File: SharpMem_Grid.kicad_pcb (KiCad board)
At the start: 2 copper layers, 45 x 36 mm, 33 parts, among them J1 CONN_01X05, J2 CONN_01X01, J3 CONN_01X01, P1 USB_B, P2 CONN_02X04, SW1 PTS810_SJK_250_SMTR_LFS, SW2 PTS810_SJK_250_SMTR_LFS, U1 25LC_EEPROM, U2 Schmitt_Inverter_Single, U3 PIC32MX250F128B-I/SS, Y1 ECS-080-18-23G-JGN-TR

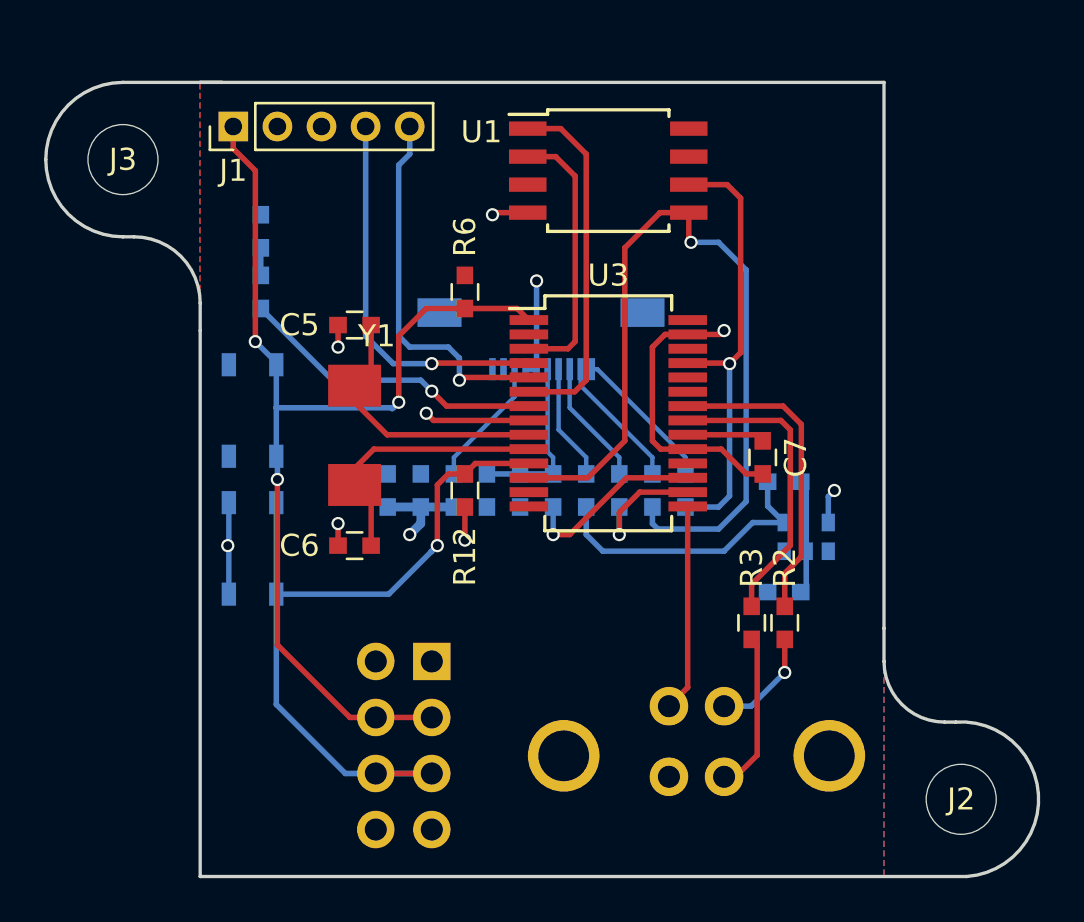
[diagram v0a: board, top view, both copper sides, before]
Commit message: redesighn for itp camp
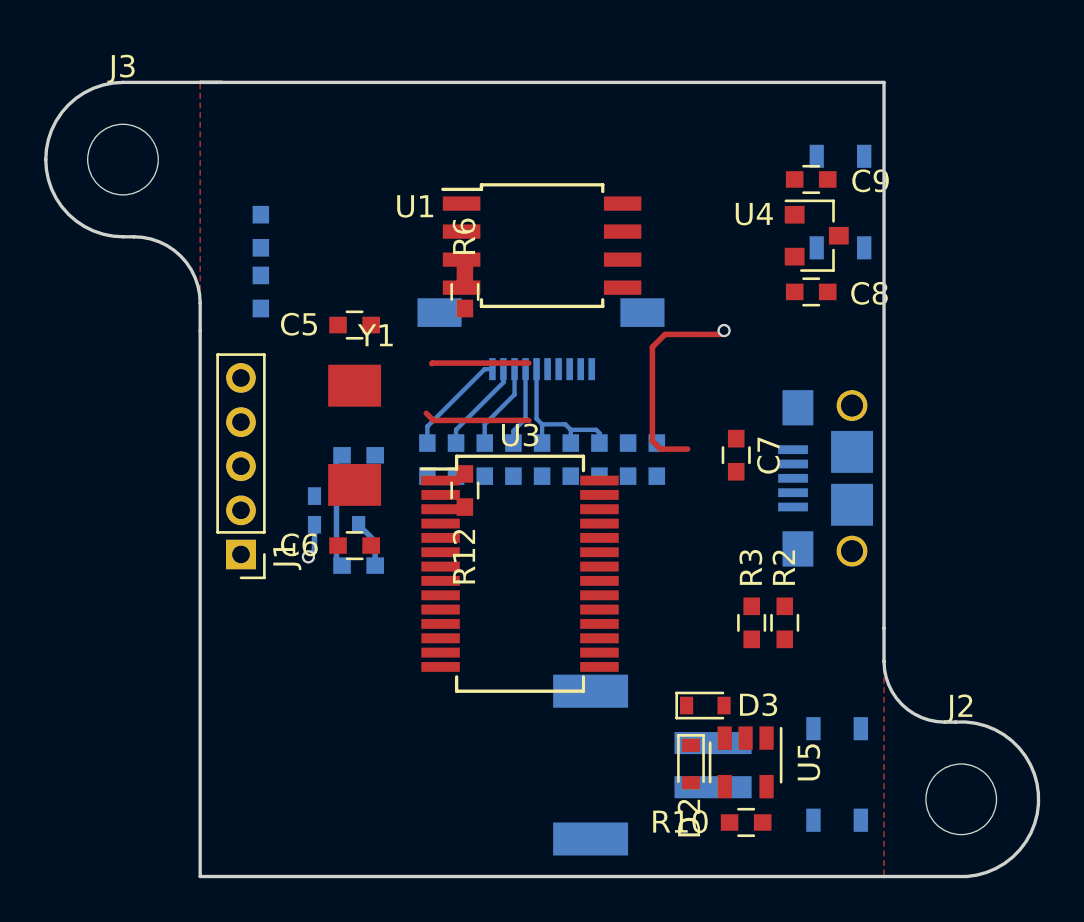
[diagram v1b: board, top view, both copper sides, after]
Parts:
- removed P1: USB_B, Solutions:USB_B_VERTICAL
- removed P2: CONN_02X04, Pin_Headers:Pin_Header_Straight_2x04_Pitch2.54mm
- added BT1: Battery_Cell, Solutions:4UCON-0217-20519, B.Cu at (184.8, 109.7)
- added C8: 1uF, Capacitors_SMD:C_0603, F.Cu at (189.2, 88.2)
- added C9: 1uF, Capacitors_SMD:C_0603, F.Cu at (189.2, 83.2)
- added D2: DIODE, Diodes_SMD:D_0603, F.Cu at (183.8, 109.7)
- added D3: DIODE, Diodes_SMD:D_0603, F.Cu at (184.4, 107.0)
- added J4: USB_B_Micro, Solutions:10118193_microUSB, B.Cu at (191.1, 96.7)
- added U4: TLV76033DBZR, TO_SOT_Packages_SMD:SOT-23, F.Cu at (189.4, 85.7)
- added U5: MCP73831-2-OT, TO_SOT_Packages_SMD:SOT-23-5, F.Cu at (186.2, 109.6)
- J2, J3: footprint Solutions:NPT_125mil -> Mounting_Holes:MountingHole_3.2mm_M3
- R10: moved to F.Cu
- R13: value 10K -> 220R
- R4, R5, R7, R8, R9: value 220 -> 220R
- moved SW2 28.4 mm to (190.0, 109.2)
- moved SW1 28.3 mm to (190.2, 83.3)
- moved U2 21.3 mm to (167.7, 98.2), turned to 270 degrees
- moved C1 20.3 mm to (168.7, 95.7), turned to 180 degrees
- moved R10 20.1 mm to (186.2, 112.3), turned to 180 degrees
- moved R1 19.7 mm to (168.7, 100.7), turned to 0 degrees
- moved J1 19.4 mm to (163.3, 100.2), turned to 180 degrees
- moved C2 12.3 mm to (182.2, 95.8), turned to 270 degrees
- moved R4 11.8 mm to (171.8, 95.8)
- moved C3 9.50 mm to (180.9, 95.8), turned to 270 degrees
- moved R5 9.01 mm to (173.1, 95.8)
- moved U3 8.30 mm to (176.0, 101.0)
- moved R7 6.26 mm to (174.4, 95.8)
- moved C4 5.29 mm to (179.6, 95.8)
- moved U1 4.53 mm to (177.0, 86.2)
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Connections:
- D1 pad 2: /LED -> /PGD
- DIS1 pad 1: GND -> Net-(DIS1-Pad1)
- DIS1 pad 10: Net-(DIS1-Pad10) -> GND
- DIS1 pad 2: GND -> Net-(DIS1-Pad2)
- DIS1 pad 4: +3V3 -> Net-(DIS1-Pad4)
- DIS1 pad 5: +3V3 -> Net-(C4-Pad1)
- DIS1 pad 6: Net-(C4-Pad1) -> +3V3
- DIS1 pad 7: Net-(DIS1-Pad7) -> +3V3
- DIS1 pad 8: Net-(DIS1-Pad8) -> +3V3
- DIS1 pad 9: Net-(DIS1-Pad9) -> GND
- R10 pad 1: Net-(DIS1-Pad3) -> Net-(R10-Pad1)
- R10 pad 2: +3V3 -> GND
- R2 pad 1: /D- -> /D+
- R3 pad 1: /D+ -> /D-
- R4 pad 1: Net-(DIS1-Pad10) -> Net-(DIS1-Pad1)
- R5 pad 1: Net-(DIS1-Pad9) -> Net-(DIS1-Pad2)
- R7 pad 1: Net-(DIS1-Pad8) -> Net-(DIS1-Pad3)
- R8 pad 1: Net-(DIS1-Pad7) -> Net-(DIS1-Pad4)
- U3 pad 7: /LED -> Net-(U3-Pad7)
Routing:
- net /MCLR: track 49.7 -> 0.00 mm, vias 3 -> 0
- net /MOSI: track 37.9 -> 0.00 mm, vias 1 -> 0
- net /PROG: track 35.6 -> 0.00 mm, vias 1 -> 0
- net /SCLK: track 20.5 -> 0.00 mm, vias 1 -> 0
- net /PGC: track 17.1 -> 0.00 mm, vias 1 -> 0
- net /EE_SS: track 16.2 -> 0.00 mm
- net /D-: track 14.1 -> 0.00 mm
- net /LED: track 14.0 -> 0.00 mm, vias 1 -> 0
- net /D+: track 13.6 -> 0.00 mm
- net +3V3: track 14.7 -> 1.57 mm, vias 4 -> 1
- net /PGD: track 17.4 -> 4.41 mm, vias 1 -> 0
- net /MISO: track 12.3 -> 0.00 mm
- net Net-(C6-Pad1): track 11.6 -> 0.00 mm
- net Net-(C5-Pad1): track 11.6 -> 0.00 mm
- net /EXTCOMIN: track 13.2 -> 2.16 mm
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- removed copper zone on B.Cu, net GND
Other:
- board text added: "Heart Bone"
- board text added: "Solutions Design & Prototyping, Brooklyn www.github.com/biomurph/SharpMem_Grid"
